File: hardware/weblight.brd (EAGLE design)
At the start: 43.2 x 12.7 mm, 16 parts, among them U1 ATtiny85-20SU

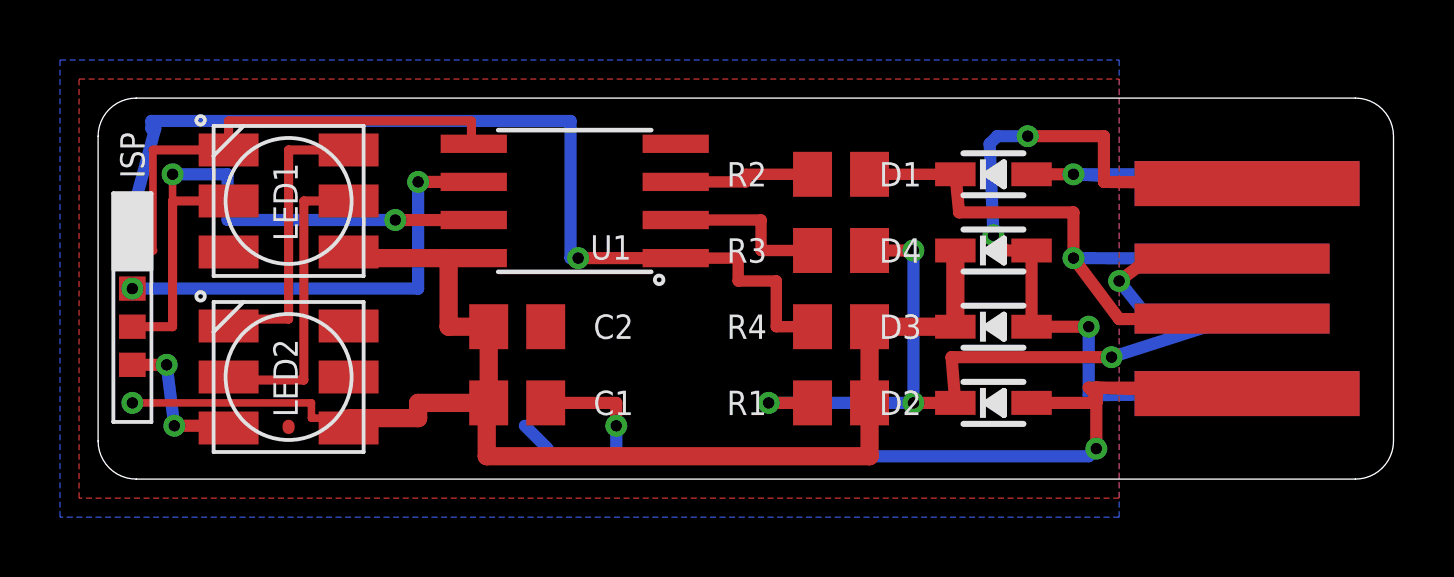
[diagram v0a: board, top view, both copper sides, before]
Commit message: Mitering
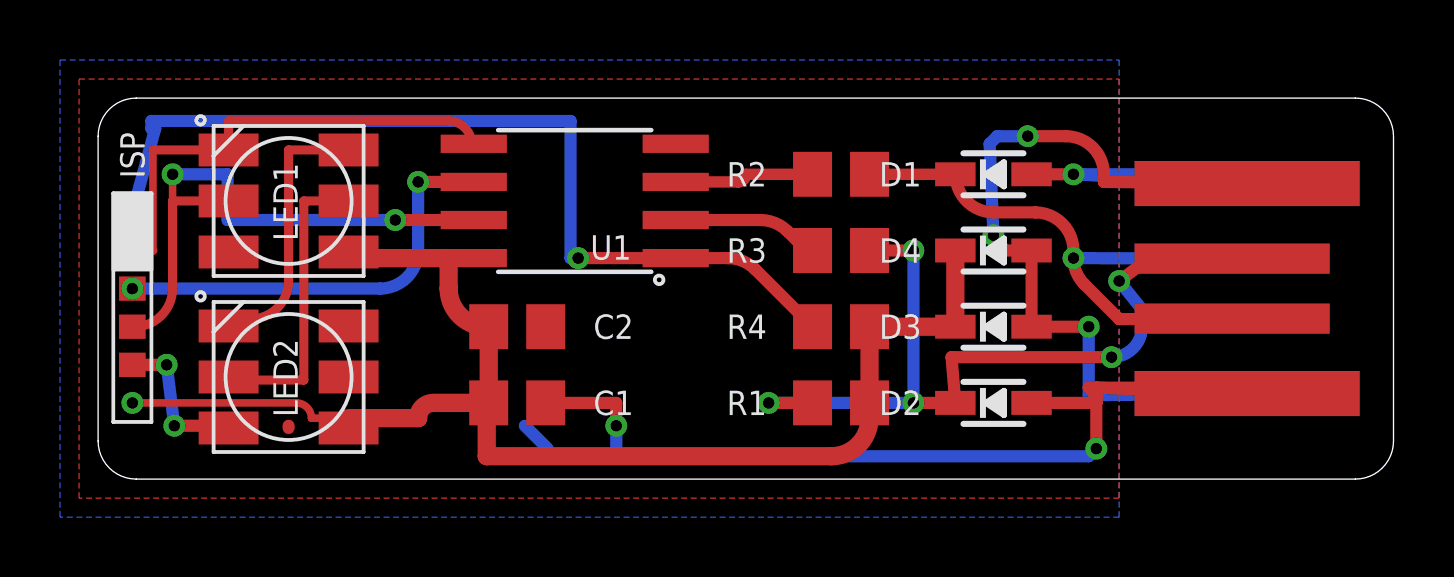
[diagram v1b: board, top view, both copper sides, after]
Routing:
- net VCC: track 52.3 -> 50.3 mm
- net N_RESET: track 32.2 -> 30.8 mm
- net USB_D_PLUS_RAW: track 21.1 -> 19.8 mm
- net 5V: track 26.8 -> 26.1 mm
- net MISO: track 14.9 -> 14.2 mm
- net DIN_2: track 9.87 -> 9.12 mm
- net CLK_1/SCK: track 19.9 -> 19.1 mm
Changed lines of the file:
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@@
 <wire x1="13.02" y1="2.54" x2="12.954" y2="2.54" width="0.381" layer="1"/>
 <wire x1="12.954" y1="2.54" x2="12.954" y2="0.762" width="0.6096" layer="1"/>
-<wire x1="25.715" y1="0.762" x2="25.715" y2="2.54" width="0.6096" layer="1"/>
-<wire x1="13.02" y1="5.08" x2="11.684" y2="5.08" width="0.6096" layer="1"/>
-<wire x1="11.684" y1="5.08" x2="11.684" y2="7.366" width="0.6096" layer="1"/>
+<wire x1="12.954" y1="0.762" x2="24.445" y2="0.762" width="0.6096" layer="1"/>
+<wire x1="24.445" y1="0.762" x2="25.715" y2="2.032" width="0.6096" layer="1" curve="90"/>
+<wire x1="25.715" y1="2.032" x2="25.715" y2="2.54" width="0.6096" layer="1"/>
+<wire x1="13.02" y1="5.08" x2="12.954" y2="5.08" width="0.6096" layer="1"/>
+<wire x1="12.954" y1="5.08" x2="11.684" y2="6.35" width="0.6096" layer="1" curve="-90"/>
+<wire x1="11.684" y1="6.35" x2="11.684" y2="7.366" width="0.6096" layer="1"/>
 <wire x1="11.684" y1="7.366" x2="12.5222" y2="7.366" width="0.381" layer="1"/>
 <wire x1="11.684" y1="7.366" x2="8.35" y2="7.366" width="0.6096" layer="1"/>
 <wire x1="8.35" y1="7.366" x2="8.35" y2="7.571" width="0.381" layer="1"/>
-<wire x1="12.954" y1="2.54" x2="10.668" y2="2.54" width="0.6096" layer="1"/>
-<wire x1="10.668" y1="2.54" x2="10.668" y2="2.032" width="0.6096" layer="1"/>
+<wire x1="12.954" y1="2.54" x2="11.176" y2="2.54" width="0.6096" layer="1"/>
+<wire x1="11.176" y1="2.54" x2="10.668" y2="2.032" width="0.6096" layer="1" curve="90"/>
 <wire x1="10.668" y1="2.032" x2="8.35" y2="2.032" width="0.6096" layer="1"/>
 <wire x1="8.35" y1="2.032" x2="8.35" y2="1.7036" width="0.381" layer="1"/>
 <wire x1="13.02" y1="5.08" x2="13.02" y2="2.54" width="0.6096" layer="1"/>
 <wire x1="8.35" y1="2.032" x2="7.112" y2="2.032" width="0.254" layer="1"/>
-<wire x1="7.112" y1="2.032" x2="7.112" y2="2.54" width="0.254" layer="1"/>
-<wire x1="7.112" y1="2.54" x2="1.143" y2="2.54" width="0.254" layer="1"/>
+<wire x1="7.112" y1="2.032" x2="6.604" y2="2.54" width="0.254" layer="1" curve="90"/>
+<wire x1="6.604" y1="2.54" x2="1.143" y2="2.54" width="0.254" layer="1"/>
 <wire x1="13.02" y1="5.08" x2="12.954" y2="0.762" width="0.4064" layer="1"/>
-<wire x1="12.954" y1="0.762" x2="25.715" y2="0.762" width="0.6096" layer="1"/>
 </signal>
 <signal name="GND">
@@
 <contactref element="R3" pad="2"/>
 <contactref element="U1" pad="2"/>
-<wire x1="23.815" y1="7.62" x2="22.098" y2="7.62" width="0.381" layer="1"/>
-<wire x1="22.098" y1="7.62" x2="22.098" y2="8.636" width="0.381" layer="1"/>
-<wire x1="22.098" y1="8.636" x2="19.2532" y2="8.636" width="0.381" layer="1"/>
+<wire x1="23.815" y1="7.62" x2="23.622" y2="7.62" width="0.381" layer="1"/>
+<wire x1="19.558" y1="8.636" x2="19.2532" y2="8.636" width="0.381" layer="1"/>
+<wire x1="23.622" y1="7.62" x2="22.977975" y2="8.264025" width="0.4064" layer="1"/>
+<wire x1="22.977975" y1="8.264025" x2="22.07995" y2="8.636" width="0.4064" layer="1" curve="45"/>
+<wire x1="22.07995" y1="8.636" x2="19.2532" y2="8.636" width="0.4064" layer="1"/>
 </signal>
 <signal name="USB_D_MINUS_RAW">
@@
 <wire x1="34.036" y1="6.604" x2="35.052" y2="5.334" width="0.4064" layer="16"/>
 <wire x1="35.052" y1="5.334" x2="37.8" y2="5.35" width="0.4064" layer="16"/>
-<wire x1="37.8" y1="5.35" x2="33.782" y2="4.064" width="0.4064" layer="16"/>
+<wire x1="37.8" y1="5.35" x2="34.798" y2="5.334" width="0.4064" layer="16"/>
+<wire x1="34.798" y1="5.334" x2="34.798" y2="5.08" width="0.4064" layer="16"/>
+<wire x1="34.798" y1="5.08" x2="33.782" y2="4.064" width="0.4064" layer="16" curve="-90"/>
 <via x="33.782" y="4.064" extent="1-16" drill="0.381"/>
 <wire x1="33.782" y1="4.064" x2="28.448" y2="4.064" width="0.4064" layer="1"/>
@@
 <wire x1="37.8" y1="7.35" x2="32.512" y2="7.366" width="0.4064" layer="16"/>
 <via x="32.512" y="7.366" extent="1-16" drill="0.381"/>
-<wire x1="32.512" y1="7.366" x2="34.036" y2="5.334" width="0.4064" layer="1"/>
-<wire x1="34.036" y1="5.334" x2="37.8" y2="5.35" width="0.4064" layer="1"/>
-<wire x1="32.512" y1="7.366" x2="32.512" y2="8.89" width="0.4064" layer="1"/>
-<wire x1="32.512" y1="8.89" x2="28.702" y2="8.89" width="0.4064" layer="1"/>
-<wire x1="28.702" y1="8.89" x2="28.575" y2="10.16" width="0.4064" layer="1"/>
+<wire x1="32.512" y1="7.366" x2="32.512" y2="7.62" width="0.4064" layer="1"/>
+<wire x1="32.512" y1="7.62" x2="31.242" y2="8.89" width="0.4064" layer="1" curve="90"/>
+<wire x1="31.242" y1="8.89" x2="29.851334375" y2="8.89" width="0.4064" layer="1"/>
+<wire x1="29.851334375" y1="8.89" x2="28.5876375" y2="10.033625" width="0.4064" layer="1" curve="-84.289168"/>
+<wire x1="28.5876375" y1="10.033625" x2="28.575" y2="10.16" width="0.4064" layer="1"/>
+<wire x1="37.8" y1="5.35" x2="37.761371875" y2="5.334" width="0.4064" layer="1" curve="-45"/>
+<wire x1="37.761371875" y1="5.334" x2="34.036" y2="5.334" width="0.4064" layer="1"/>
+<wire x1="34.036" y1="5.334" x2="32.871209375" y2="6.498790625" width="0.4064" layer="1"/>
+<wire x1="32.871209375" y1="6.498790625" x2="32.512" y2="7.366" width="0.4064" layer="1" curve="-45"/>
 </signal>
 <signal name="USB_D_PLUS">
@@
 <contactref element="U1" pad="3"/>
 <wire x1="23.815" y1="10.16" x2="21.59" y2="10.16" width="0.381" layer="1"/>
-<wire x1="21.59" y1="10.16" x2="21.59" y2="9.906" width="0.381" layer="1"/>
-<wire x1="21.59" y1="9.906" x2="19.2532" y2="9.906" width="0.381" layer="1"/>
+<wire x1="21.59" y1="10.16" x2="21.336" y2="9.906" width="0.381" layer="1" curve="-90"/>
+<wire x1="21.336" y1="9.906" x2="19.2532" y2="9.906" width="0.381" layer="1"/>
 </signal>
 <signal name="N_RESET">
@@
 <contactref element="ISP" pad="1"/>
 <contactref element="U1" pad="1"/>
-<wire x1="23.815" y1="5.08" x2="22.606" y2="5.08" width="0.381" layer="1"/>
-<wire x1="22.606" y1="5.08" x2="22.606" y2="6.604" width="0.381" layer="1"/>
-<wire x1="22.606" y1="6.604" x2="21.336" y2="6.604" width="0.381" layer="1"/>
-<wire x1="21.336" y1="6.604" x2="21.336" y2="7.366" width="0.381" layer="1"/>
-<wire x1="21.336" y1="7.366" x2="19.2532" y2="7.366" width="0.381" layer="1"/>
 <wire x1="19.2532" y1="7.366" x2="16.002" y2="7.366" width="0.4064" layer="1"/>
 <via x="16.002" y="7.366" extent="1-16" drill="0.381"/>
@@
 <wire x1="1.778" y1="11.684" x2="1.905" y2="11.684" width="0.4064" layer="16"/>
 <wire x1="1.905" y1="11.684" x2="1.143" y2="8.89" width="0.4064" layer="16"/>
+<wire x1="23.815" y1="5.08" x2="21.900975" y2="6.994025" width="0.4064" layer="1"/>
+<wire x1="21.900975" y1="6.994025" x2="21.00295" y2="7.366" width="0.4064" layer="1" curve="45"/>
+<wire x1="21.00295" y1="7.366" x2="19.2532" y2="7.366" width="0.4064" layer="1"/>
 </signal>
 <signal name="CLK_1/SCK">
@@
 <contactref element="ISP" pad="4"/>
 <wire x1="4.35" y1="9.271" x2="2.48285" y2="9.271" width="0.3048" layer="1"/>
-<wire x1="2.48285" y1="9.271" x2="2.48285" y2="5.08" width="0.3048" layer="1"/>
-<wire x1="2.48285" y1="5.08" x2="1.143" y2="5.08" width="0.3048" layer="1"/>
+<wire x1="2.48285" y1="9.271" x2="2.48285" y2="6.35" width="0.3048" layer="1"/>
+<wire x1="2.48285" y1="6.35" x2="1.21285" y2="5.08" width="0.3048" layer="1" curve="-90"/>
+<wire x1="1.21285" y1="5.08" x2="1.143" y2="5.08" width="0.3048" layer="1"/>
 <wire x1="12.5222" y1="8.636" x2="9.906" y2="8.636" width="0.4064" layer="1"/>
 <via x="9.906" y="8.636" extent="1-16" drill="0.381"/>
@@
 <contactref element="LED2" pad="DI"/>
 <wire x1="8.35" y1="10.971" x2="6.35" y2="10.971" width="0.3048" layer="1"/>
-<wire x1="6.35" y1="10.971" x2="6.35" y2="5.334" width="0.3048" layer="1"/>
-<wire x1="6.35" y1="5.334" x2="4.35" y2="5.334" width="0.3048" layer="1"/>
+<wire x1="6.35" y1="10.971" x2="6.35" y2="6.604" width="0.3048" layer="1"/>
+<wire x1="6.35" y1="6.604" x2="5.08" y2="5.334" width="0.3048" layer="1" curve="-90"/>
+<wire x1="5.08" y1="5.334" x2="4.35" y2="5.334" width="0.3048" layer="1"/>
 <wire x1="4.35" y1="5.334" x2="4.35" y2="5.1036" width="0.3048" layer="1"/>
 </signal>
@@
 <wire x1="12.5222" y1="9.906" x2="10.668" y2="9.906" width="0.4064" layer="1"/>
 <via x="10.668" y="9.906" extent="1-16" drill="0.381"/>
-<wire x1="10.668" y1="9.906" x2="10.668" y2="6.35" width="0.4064" layer="16"/>
-<wire x1="10.668" y1="6.35" x2="1.143" y2="6.35" width="0.4064" layer="16"/>
+<wire x1="10.668" y1="9.906" x2="10.668" y2="7.62" width="0.4064" layer="16"/>
+<wire x1="10.668" y1="7.62" x2="9.398" y2="6.35" width="0.4064" layer="16" curve="-90"/>
+<wire x1="9.398" y1="6.35" x2="1.143" y2="6.35" width="0.4064" layer="16"/>
 <via x="1.143" y="6.35" extent="1-16" drill="0.381"/>
 </signal>
@@
 <contactref element="U1" pad="5"/>
 <wire x1="12.5222" y1="11.176" x2="12.446" y2="11.176" width="0.3048" layer="1"/>
-<wire x1="12.446" y1="11.176" x2="12.446" y2="11.938" width="0.3048" layer="1"/>
-<wire x1="12.446" y1="11.938" x2="4.35" y2="11.938" width="0.3048" layer="1"/>
+<wire x1="12.446" y1="11.176" x2="11.684" y2="11.938" width="0.3048" layer="1" curve="90"/>
+<wire x1="11.684" y1="11.938" x2="4.35" y2="11.938" width="0.3048" layer="1"/>
 <wire x1="4.35" y1="11.938" x2="4.35" y2="10.971" width="0.3048" layer="1"/>
 <wire x1="4.35" y1="10.971" x2="1.8288" y2="10.971" width="0.3048" layer="1"/>
@@
 <wire x1="33.02" y1="5.08" x2="31.115" y2="5.08" width="0.4064" layer="1"/>
 <wire x1="38.3" y1="9.85" x2="33.528" y2="9.906" width="0.4064" layer="1"/>
-<wire x1="33.528" y1="9.906" x2="33.528" y2="11.43" width="0.4064" layer="1"/>
-<wire x1="33.528" y1="11.43" x2="30.988" y2="11.43" width="0.4064" layer="1"/>
+<wire x1="33.528" y1="9.906" x2="33.528" y2="10.16" width="0.4064" layer="1"/>
+<wire x1="33.528" y1="10.16" x2="32.258" y2="11.43" width="0.4064" layer="1" curve="90"/>
+<wire x1="32.258" y1="11.43" x2="30.988" y2="11.43" width="0.4064" layer="1"/>
 <via x="30.988" y="11.43" extent="1-16" drill="0.381"/>
 <wire x1="30.988" y1="11.43" x2="29.972" y2="11.43" width="0.4064" layer="16"/>
